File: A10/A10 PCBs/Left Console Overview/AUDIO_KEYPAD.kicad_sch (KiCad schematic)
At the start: 24 parts, among them J36 AUDIO_KEYPAD, SW50 LOAD, SW51 LOAD, SW52 LOAD, SW53 LOAD, SW54 LOAD, SW55 LOAD, SW56 LOAD, SW57 LOAD, SW58 LOAD, SW59 LOAD, SW60 LOAD, SW61 LOAD, SW62 ESC, SW63 INTERCOMM, SW64 VHF, SW65 ARM

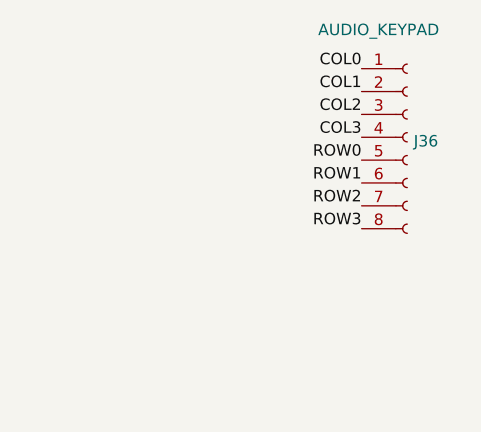
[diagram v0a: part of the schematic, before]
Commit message: A10
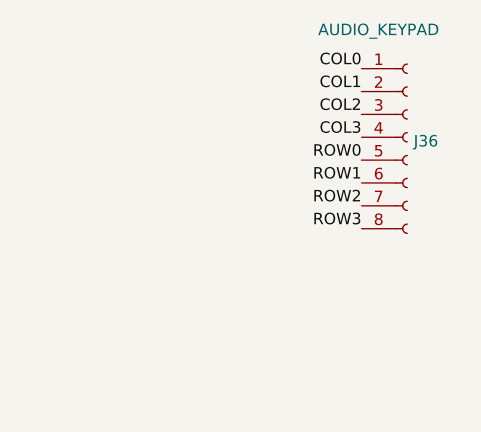
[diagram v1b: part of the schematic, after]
